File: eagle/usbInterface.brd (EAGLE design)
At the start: 40 x 20 mm, 22 parts

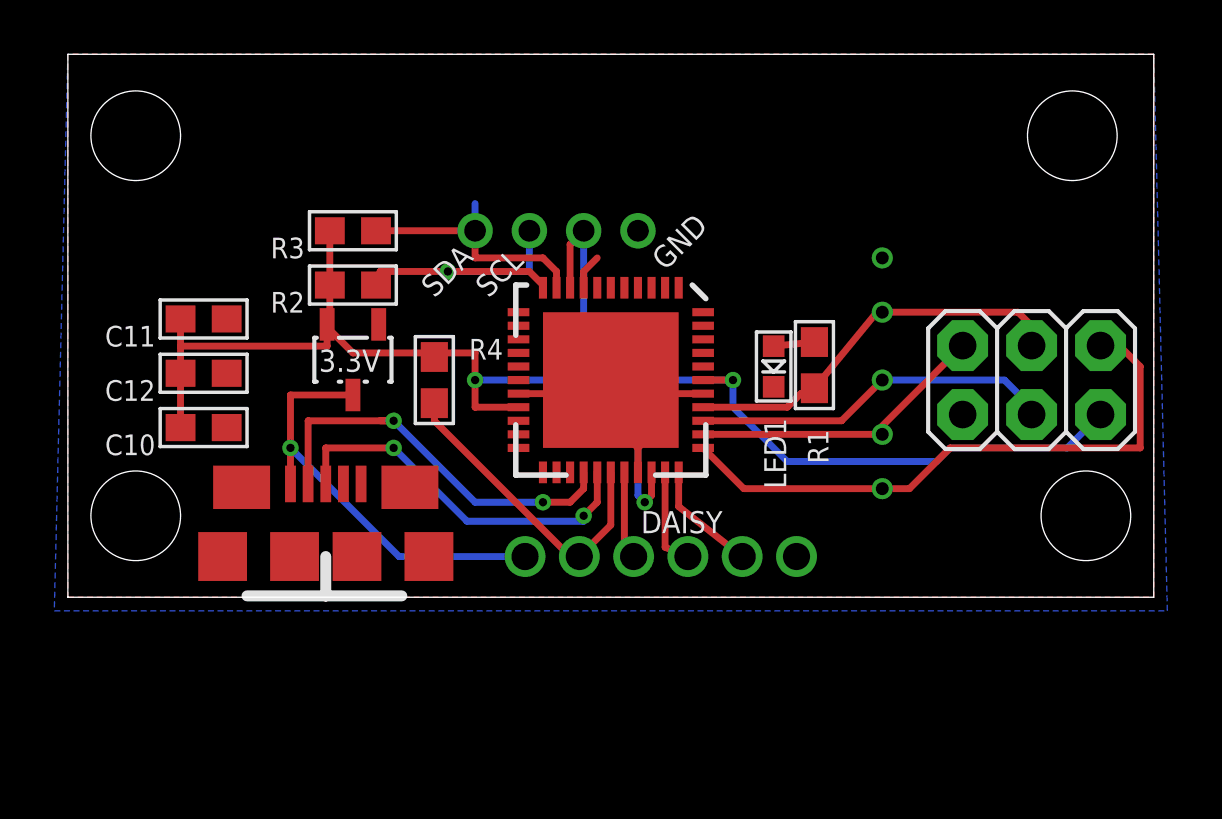
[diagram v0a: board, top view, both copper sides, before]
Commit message: added up to date usb interface board
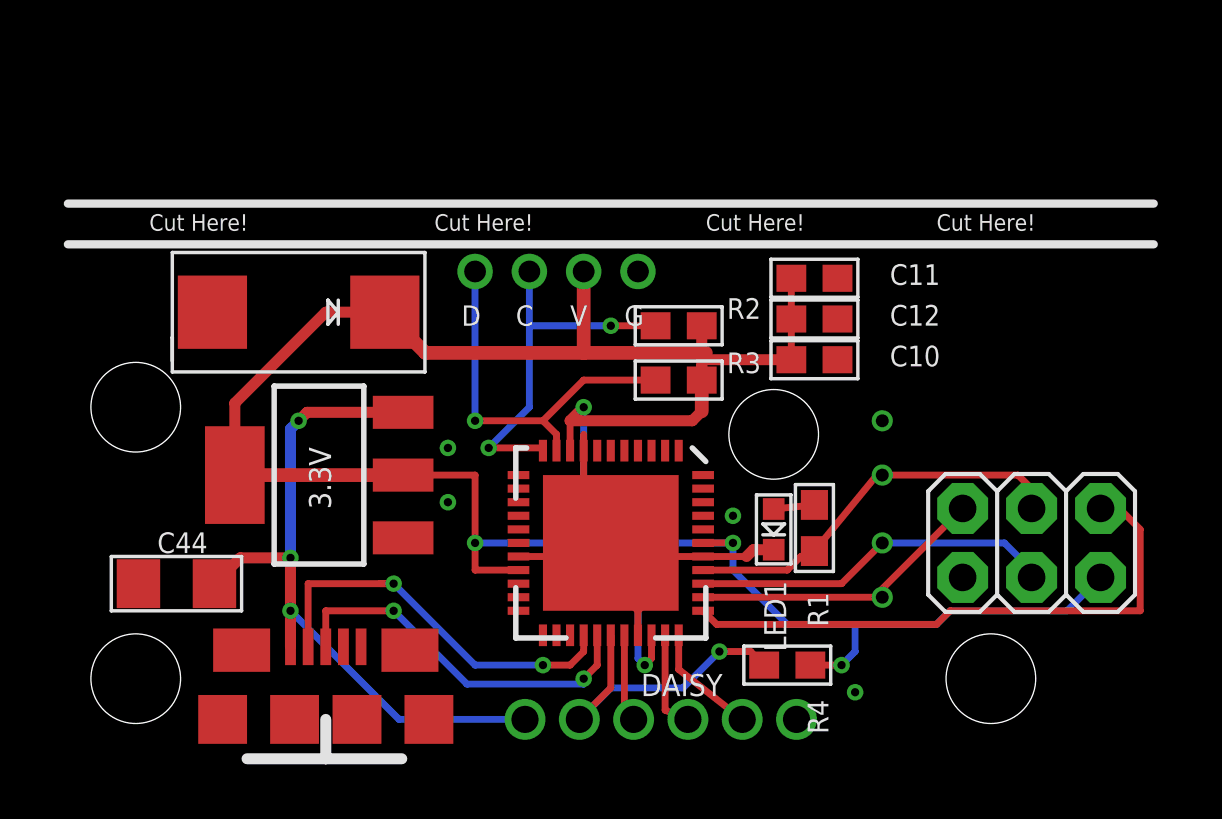
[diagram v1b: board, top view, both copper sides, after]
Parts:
- added C43: 470uF, microbuilder:EIA7343-31/D-R
- added C44: 10uF, nonolith:1206
- 3.3V: value VREG -> VREGAP1117; device nonolith:SOT23-3 -> nonolith:SOT223
- moved C10 22.6 mm to (7.50, 8.75)
- moved C12 22.6 mm to (7.50, 10.2)
- moved C11 22.5 mm to (7.50, 11.8)
- moved R4 16.7 mm to (6.50, -2.50), turned to 0 degrees
- moved U$4 15.6 mm to (6.00, 6.00)
- moved R3 13.2 mm to (2.50, 8.00), turned to 0 degrees
- moved R2 12.1 mm to (2.50, 10.0), turned to 0 degrees
- moved U$3 10.0 mm to (-17.5, 7.00)
- moved U$2 6.95 mm to (14.0, -3.00)
- moved R1 6.00 mm to (7.50, 2.55)
- moved CN1 6.00 mm to (-10.5, -4.50)
- moved DAISY 6.00 mm to (7.00, -4.50)
- moved LED1 6.00 mm to (6.00, 2.50)
- moved PROGX 6.00 mm to (15.5, 2.00)
- moved U$1 6.00 mm to (-17.5, -3.00)
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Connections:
- net 3.3V: now also 3.3V.4, C43.+
- net 5V: now also C44.2
- net GND: now also C43.-, C44.1
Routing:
- net 3.3V: track 63.7 -> 95.8 mm, vias 3 -> 5
- net 5V: track 15.9 -> 25.9 mm, vias 1 -> 3
- net GND: track 11.2 -> 17.1 mm, vias 1 -> 5
- net SDA: track 9.46 -> 14.1 mm, vias 0 -> 1
- net SCL: track 11.5 -> 13.9 mm, vias 1 -> 2
- net PDI-DATA: track 22.1 -> 21.3 mm, vias 1 -> 0
- net PE0: track 11.6 -> 12.0 mm, vias 0 -> 1
- removed copper zone on layer 1, net GND
- removed copper zone on layer 16, net GND
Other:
- board outline removed
- board text added: "C"
- board text added: "Cut Here!"
- board text added: "D"
- board text added: "G"
- board text added: "V"
- board text removed: "GND"
- board text removed: "SCL"
- board text removed: "SDA"
